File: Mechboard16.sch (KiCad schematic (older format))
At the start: 154 parts, among them CN1 CONN_C16, CN2 CONN_+4, SW0:0 KEY_DEL, SW0:1 KEY_RET, SW0:2 KEY_PND, SW0:3 KEY_HLP, SW0:4 KEY_F1, SW0:5 KEY_F2, SW0:6 KEY_F3, SW0:7 KEY_AT, SW1:0 KEY_3, SW1:1 KEY_W, SW1:2 KEY_A, SW1:3 KEY_4, SW1:4 KEY_Z, SW1:5 KEY_S, SW1:6 KEY_E, SW1:7 KEY_LSH, SW1B:7 KEY_RSH, SW1C:7 KEY_CLK, SW2:0 KEY_5, SW2:1 KEY_R, SW2:2 KEY_D, SW2:3 KEY_6, SW2:4 KEY_C, SW2:5 KEY_F, SW2:6 KEY_T, SW2:7 KEY_X, SW3:0 KEY_7, SW3:1 KEY_Y, SW3:2 KEY_G, SW3:3 KEY_8, SW3:4 KEY_B, SW3:5 KEY_H, SW3:6 KEY_U, SW3:7 KEY_V, SW4:0 KEY_9, SW4:1 KEY_I, SW4:2 KEY_J, SW4:3 KEY_0, SW4:4 KEY_M, SW4:5 KEY_K, SW4:6 KEY_O, SW4:7 KEY_N, SW5:0 KEY_DN, SW5:1 KEY_P, SW5:2 KEY_L, SW5:3 KEY_UP, SW5:4 KEY_DOT, SW5:5 KEY_COL, SW5:6 KEY_MIN, SW5:7 KEY_COM, SW6:0 KEY_LF, SW6:1 KEY_AST, SW6:2 KEY_SEM, SW6:3 KEY_RT, SW6:4 KEY_ESC, SW6:5 KEY_EQ, SW6:6 KEY_PLS, SW6:7 KEY_SLA, SW7:0 KEY_1, SW7:1 KEY_CLR, SW7:2 KEY_CTL, SW7:3 KEY_2, SW7:4 KEY_SPC, SW7:5 KEY_CMD, SW7:6 KEY_Q, SW7:7 KEY_RUN, U1 4066, U2 NE555

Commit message: Routing... Routing... Routing...
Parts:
- SW0:3, SW0:4, SW0:5, SW0:6: footprint Mechboard16:SW_Hotswap_Kailh_MX_1.50u_OffsetR -> Mechboard16:SW_Hotswap_Kailh_MX_1.50u_OffsetL
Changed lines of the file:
@@
 F 0 "SW0:4" H 3705 1390 50  0000 C CNN
 F 1 "KEY_F1" V 3950 1560 50  0000 C CNN
-F 2 "Mechboard16:SW_Hotswap_Kailh_MX_1.50u_OffsetR" H 3775 1535 50  0001 C CNN
+F 2 "Mechboard16:SW_Hotswap_Kailh_MX_1.50u_OffsetL" H 3775 1535 50  0001 C CNN
 F 3 "~" H 3775 1535 50  0001 C CNN
 	1    3775 1535
@@
 F 0 "SW0:5" H 4220 1390 50  0000 C CNN
 F 1 "KEY_F2" V 4455 1570 50  0000 C CNN
-F 2 "Mechboard16:SW_Hotswap_Kailh_MX_1.50u_OffsetR" H 4275 1535 50  0001 C CNN
+F 2 "Mechboard16:SW_Hotswap_Kailh_MX_1.50u_OffsetL" H 4275 1535 50  0001 C CNN
 F 3 "~" H 4275 1535 50  0001 C CNN
 	1    4275 1535
@@
 F 0 "SW0:6" H 4700 1390 50  0000 C CNN
 F 1 "KEY_F3" V 4950 1560 50  0000 C CNN
-F 2 "Mechboard16:SW_Hotswap_Kailh_MX_1.50u_OffsetR" H 4775 1535 50  0001 C CNN
+F 2 "Mechboard16:SW_Hotswap_Kailh_MX_1.50u_OffsetL" H 4775 1535 50  0001 C CNN
 F 3 "~" H 4775 1535 50  0001 C CNN
 	1    4775 1535
@@
 F 0 "SW0:3" H 3195 1390 50  0000 C CNN
 F 1 "KEY_HLP" V 3445 1545 50  0000 C CNN
-F 2 "Mechboard16:SW_Hotswap_Kailh_MX_1.50u_OffsetR" H 3275 1535 50  0001 C CNN
+F 2 "Mechboard16:SW_Hotswap_Kailh_MX_1.50u_OffsetL" H 3275 1535 50  0001 C CNN
 F 3 "~" H 3275 1535 50  0001 C CNN
 	1    3275 1535

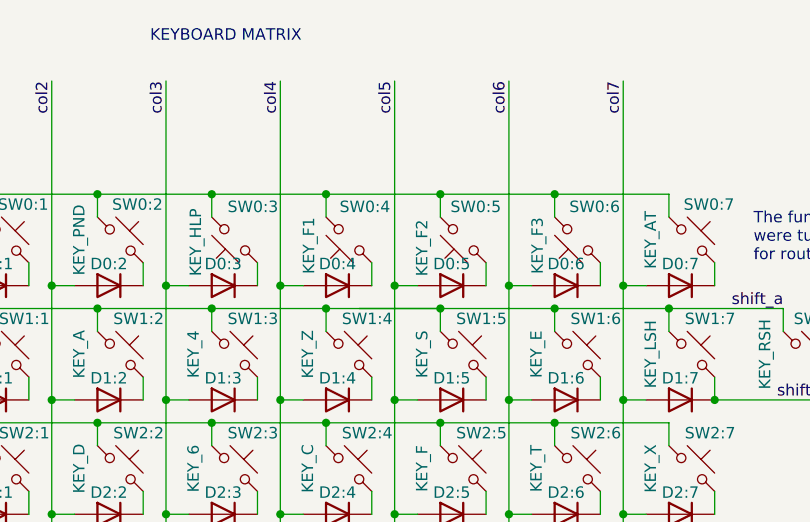
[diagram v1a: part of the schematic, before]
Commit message: -30
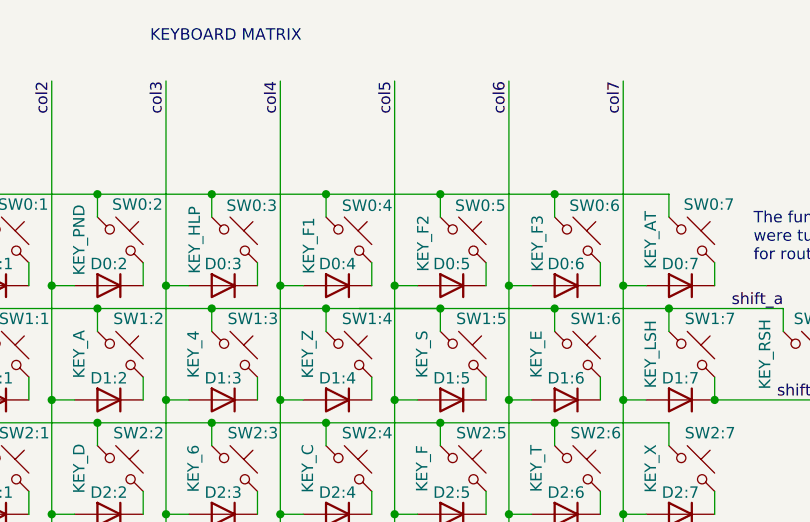
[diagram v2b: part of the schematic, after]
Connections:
- net row0: now also SW0:3.1, SW0:4.1, SW0:5.1, SW0:6.1; no longer SW0:3.2, SW0:4.2, SW0:5.2, SW0:6.2
- net at D0:3.1 (K): now also SW0:3.2; no longer SW0:3.1
- net at D0:4.1 (K): now also SW0:4.2; no longer SW0:4.1
- net at D0:5.1 (K): now also SW0:5.2; no longer SW0:5.1
- net at D0:6.1 (K): now also SW0:6.2; no longer SW0:6.1
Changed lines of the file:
@@
 Wire Wire Line
 	2975 2735 2975 3235
-$Comp
-L Switch:SW_Push_45deg SW0:4
-U 1 1 6581A489
-P 3775 1535
-F 0 "SW0:4" H 3705 1390 50  0000 C CNN
-F 1 "KEY_F1" V 3950 1560 50  0000 C CNN
-F 2 "Mechboard16:SW_Hotswap_Kailh_MX_1.50u_OffsetL" H 3775 1535 50  0001 C CNN
-F 3 "~" H 3775 1535 50  0001 C CNN
-	1    3775 1535
-	-1   0    0    1
-$EndComp
 Wire Wire Line
 	3675 1435 3675 1335
@@
 U 1 1 65838F0C
 P 4275 1535
-F 0 "SW0:5" H 4220 1390 50  0000 C CNN
-F 1 "KEY_F2" V 4455 1570 50  0000 C CNN
+F 0 "SW0:5" H 4350 1685 50  0000 C CNN
+F 1 "KEY_F2" V 4100 1520 50  0000 C CNN
 F 2 "Mechboard16:SW_Hotswap_Kailh_MX_1.50u_OffsetL" H 4275 1535 50  0001 C CNN
 F 3 "~" H 4275 1535 50  0001 C CNN
 	1    4275 1535
-	-1   0    0    1
+	1    0    0    -1
 $EndComp
 Wire Wire Line
@@
 U 1 1 6586B7F1
 P 4775 1535
-F 0 "SW0:6" H 4700 1390 50  0000 C CNN
-F 1 "KEY_F3" V 4950 1560 50  0000 C CNN
+F 0 "SW0:6" H 4850 1685 50  0000 C CNN
+F 1 "KEY_F3" V 4600 1520 50  0000 C CNN
 F 2 "Mechboard16:SW_Hotswap_Kailh_MX_1.50u_OffsetL" H 4775 1535 50  0001 C CNN
 F 3 "~" H 4775 1535 50  0001 C CNN
 	1    4775 1535
-	-1   0    0    1
+	1    0    0    -1
 $EndComp
 Wire Wire Line
@@
 U 1 1 6580578A
 P 3275 1535
-F 0 "SW0:3" H 3195 1390 50  0000 C CNN
-F 1 "KEY_HLP" V 3445 1545 50  0000 C CNN
+F 0 "SW0:3" H 3350 1685 50  0000 C CNN
+F 1 "KEY_HLP" V 3100 1535 50  0000 C CNN
 F 2 "Mechboard16:SW_Hotswap_Kailh_MX_1.50u_OffsetL" H 3275 1535 50  0001 C CNN
 F 3 "~" H 3275 1535 50  0001 C CNN
 	1    3275 1535
-	-1   0    0    1
+	1    0    0    -1
 $EndComp
 $Comp
@@
 Wire Bus Line
 	2190 5975 2190 6805
+$Comp
+L Switch:SW_Push_45deg SW0:4
+U 1 1 6581A489
+P 3775 1535
+F 0 "SW0:4" H 3855 1685 50  0000 C CNN
+F 1 "KEY_F1" V 3600 1510 50  0000 C CNN
+F 2 "Mechboard16:SW_Hotswap_Kailh_MX_1.50u_OffsetL" H 3775 1535 50  0001 C CNN
+F 3 "~" H 3775 1535 50  0001 C CNN
+	1    3775 1535
+	1    0    0    -1
+$EndComp
 $EndSCHEMATC
